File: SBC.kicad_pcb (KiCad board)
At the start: 6 copper layers, 85 x 54 mm, 284 parts, among them J1 USB_OTG, J2 Conn_ARM_JTAG_SWD_20, J3 USB_OTG, J4 Conn_02x25_Counter_Clockwise, U1 STPMIC1APQR, U2 IS43TR16640C-125JBL, U3 ECMF02-2AMX6, U4 ECMF02-2AMX6, U6 IS21ES08GA-JQLI-TR, U7 LAN8720A, U8 ARJM11C7-114-BA-EW2, U9 STM32MP153AABx, X1 ASE-24MHz, Y1 25MHz

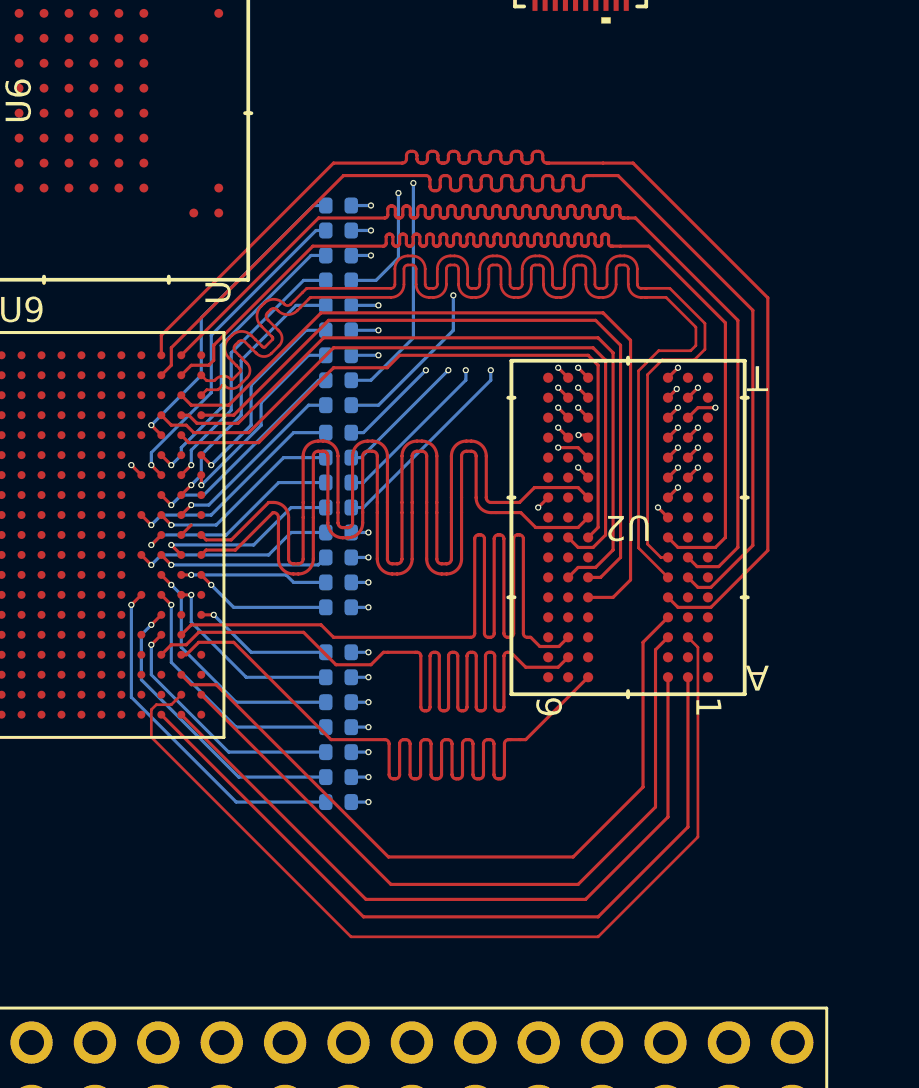
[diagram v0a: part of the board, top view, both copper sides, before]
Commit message: DDR routing
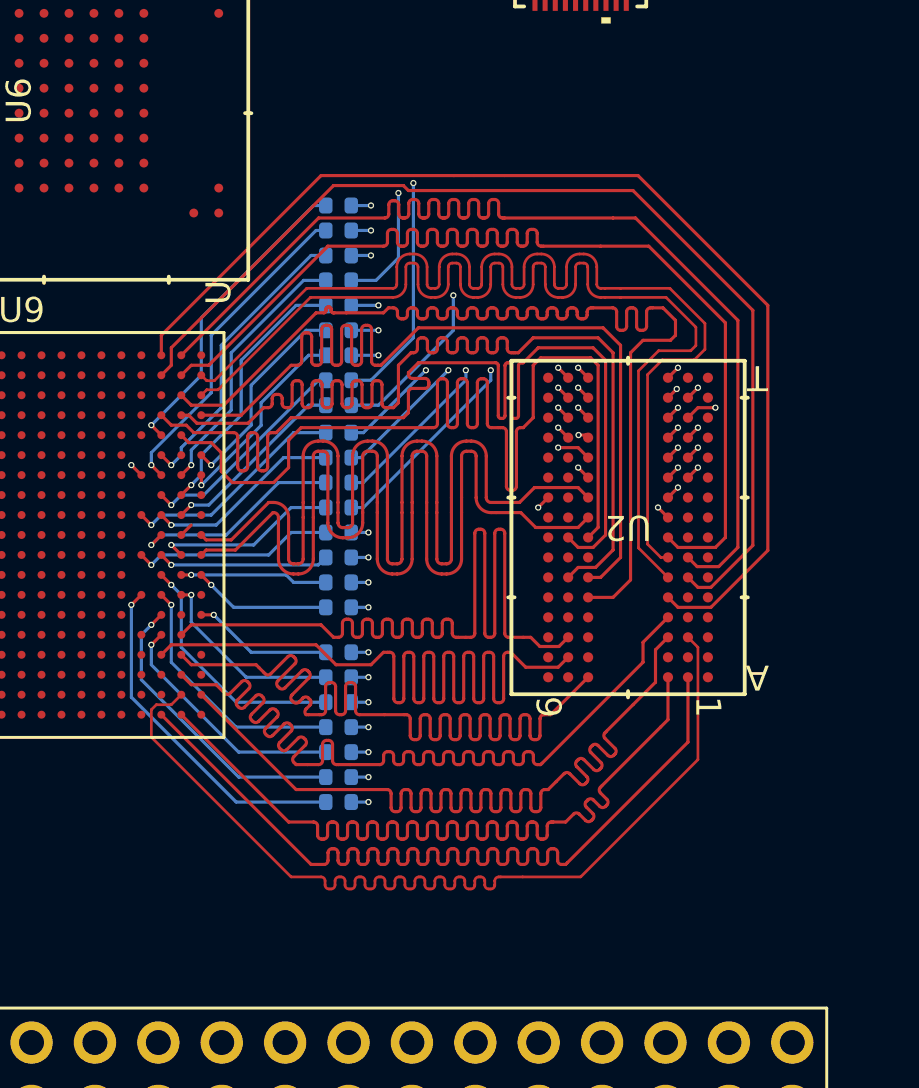
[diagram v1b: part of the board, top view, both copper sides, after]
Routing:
- net /MPU/DQ4: track 25.5 -> 44.6 mm
- net /MPU/DQ5: track 28.6 -> 44.9 mm
- net /MPU/DQ2: track 29.3 -> 44.7 mm
- net /MPU/DDR_DQM0: track 31.7 -> 44.7 mm
- net /MPU/DQ6: track 28.9 -> 39.7 mm
- net /MPU/DQ12: track 29.5 -> 39.6 mm
- net /MPU/DQ11: track 29.6 -> 39.7 mm
- net /MPU/DDR_DQM1: track 29.9 -> 39.6 mm
- net /MPU/DQ15: track 31.9 -> 39.7 mm
- net /MPU/DQ3: track 49.8 -> 42.2 mm
- net /MPU/DQ0: track 49.8 -> 44.8 mm
- net /MPU/DQ7: track 49.7 -> 44.8 mm
- net /MPU/DQ1: track 49.7 -> 44.8 mm
- net /MPU/DDR_DQS0_N: track 49.4 -> 44.5 mm
- net /MPU/DDR_DQS0_P: track 49.6 -> 44.7 mm
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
